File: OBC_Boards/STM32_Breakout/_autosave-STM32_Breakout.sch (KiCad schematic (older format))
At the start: 96 parts, among them J1 Conn_02x20_Odd_Even, J2 ST1W008S4ER1500-MicroSDConnec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, J3 1050171001, J4 105017-1001, J5 1050171001, J6 SSQ-105-03-T-D, J7 SSQ-105-03-T-D, Q1 Q_PMOS_DGS, U1 MR25H10MDF, U2 BU33SA5WGWZ-E2-qsat-symb, U3 STM32L4A6ZGT6P, U4 MCP7940NT-I_MS, U5 FSM6JSMATR, U6 MCP9808

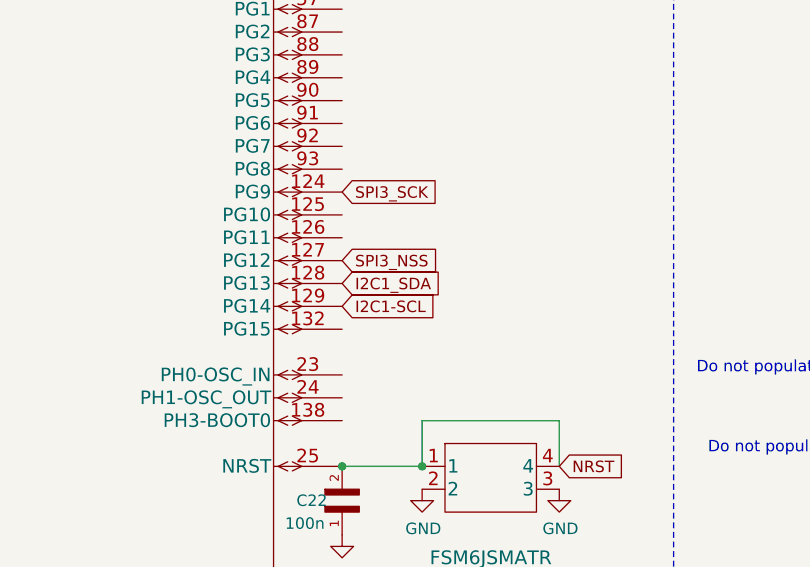
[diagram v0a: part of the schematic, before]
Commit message: First complete draft
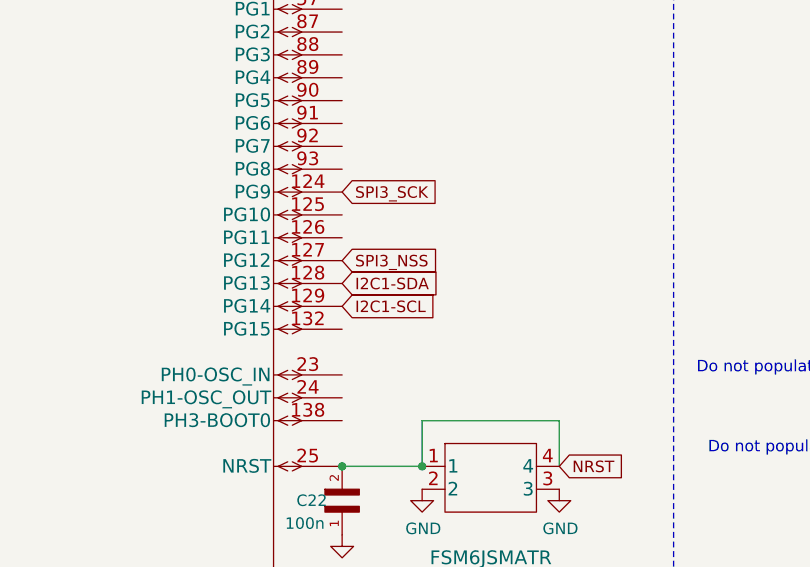
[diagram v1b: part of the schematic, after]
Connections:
- net I2C1_SDA: no longer U3.128 (PG13)
- new net I2C1-SDA: U3.128 (PG13)
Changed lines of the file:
@@
 SPI3_NSS
 Text GLabel 12950 11150 2    50   Input ~ 0
-I2C1_SDA
+I2C1-SDA
 Text GLabel 12950 11250 2    50   Input ~ 0
 I2C1-SCL
